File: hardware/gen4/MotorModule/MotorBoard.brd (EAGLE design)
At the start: 34 x 61.7 mm, 67 parts, among them IC1 XMEGA16A4A, M1O1 TEST_PT, M1O2 TEST_PT, M1O3 TEST_PT

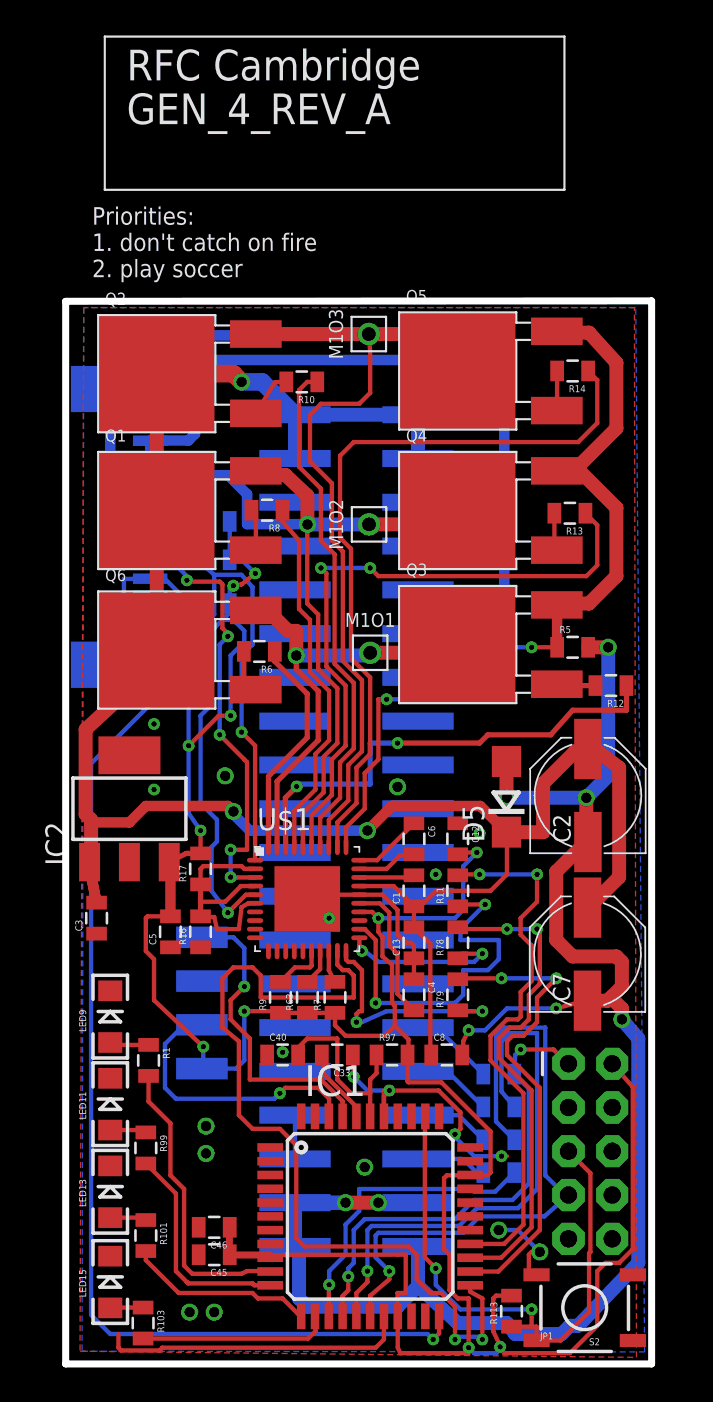
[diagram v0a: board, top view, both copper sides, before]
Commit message: fixing motorboard
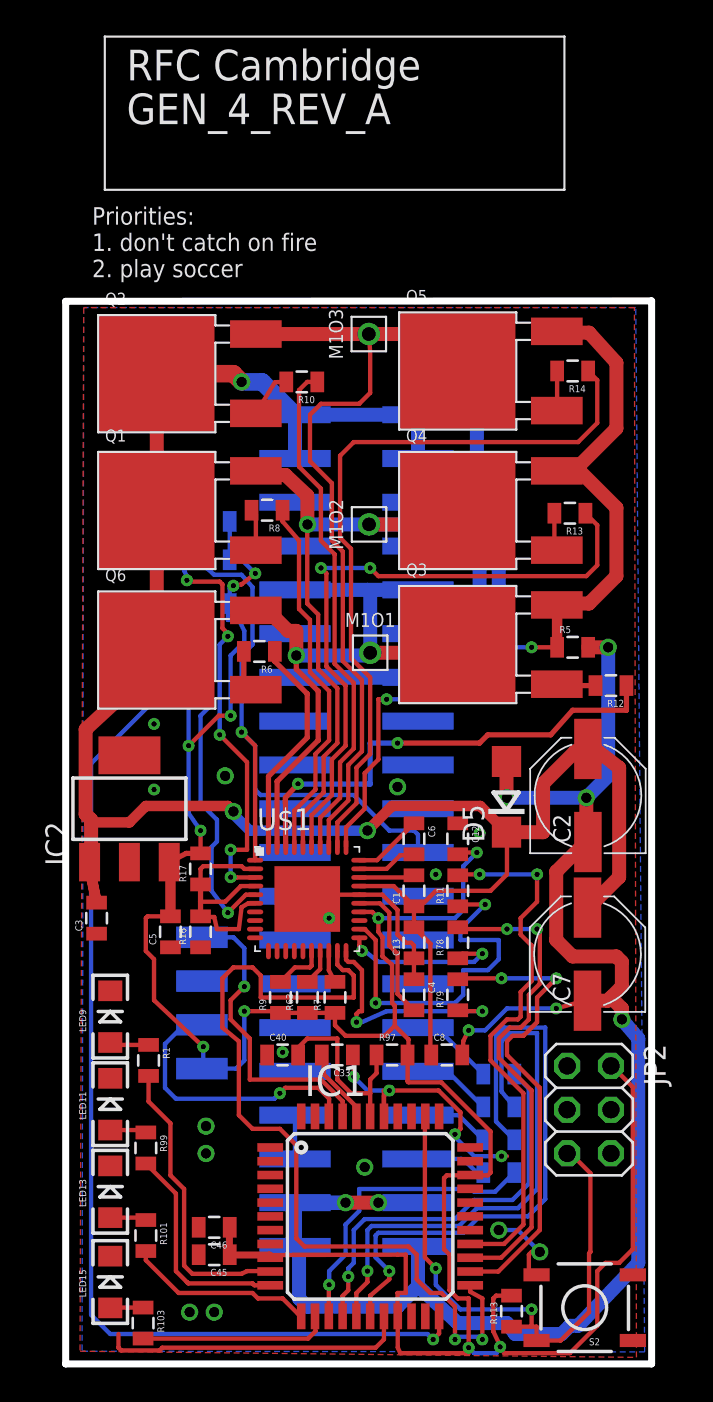
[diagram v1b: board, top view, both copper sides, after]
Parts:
- removed JP1: (no value), SparkFun-Connectors:2X5-SHROUDED-NS
- removed U$2: MOTORCON, gen3:GEN3CON
- added JP2: (no value), pinhead:2X03
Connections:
- new net DATA: IC1.34, JP2.1
- net 3.3V: now also JP2.2, JP3.23; no longer JP1.2, U$2.1
- net GND: now also JP2.6, JP3.15; no longer JP1.10, JP1.4, JP1.6, JP1.8, U$2.5
- net M1H1: now also JP3.19; no longer U$2.3
- net M1H2: now also JP3.17; no longer U$2.4
- net M1H3: now also JP3.21; no longer U$2.2
- net M1O1: now also JP3.10, JP3.9; no longer U$2.10, U$2.11
- net M1O2: now also JP3.11, JP3.12; no longer U$2.8, U$2.9
- net M1O3: now also JP3.13, JP3.14; no longer U$2.6, U$2.7
- net MOSI: no longer JP1.1
- net RESET: now also JP2.5; no longer JP1.5
- net SCK: no longer JP1.7
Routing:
- net M1O1: track 77.0 -> 37.6 mm
- net M1O3: track 76.8 -> 91.4 mm
- net M1H1: track 31.5 -> 23.0 mm
- net M1H3: track 28.1 -> 35.7 mm
- net 3.3V: track 159.9 -> 154.5 mm
- net MOSI: track 28.0 -> 23.3 mm, vias 2 -> 1
- net M1O2: track 49.0 -> 51.9 mm
- net M1H2: track 28.3 -> 26.3 mm
- net SCK: track 37.6 -> 35.7 mm
